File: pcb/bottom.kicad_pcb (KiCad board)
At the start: 2 copper layers, 128.6 x 95.2 mm, 7 parts

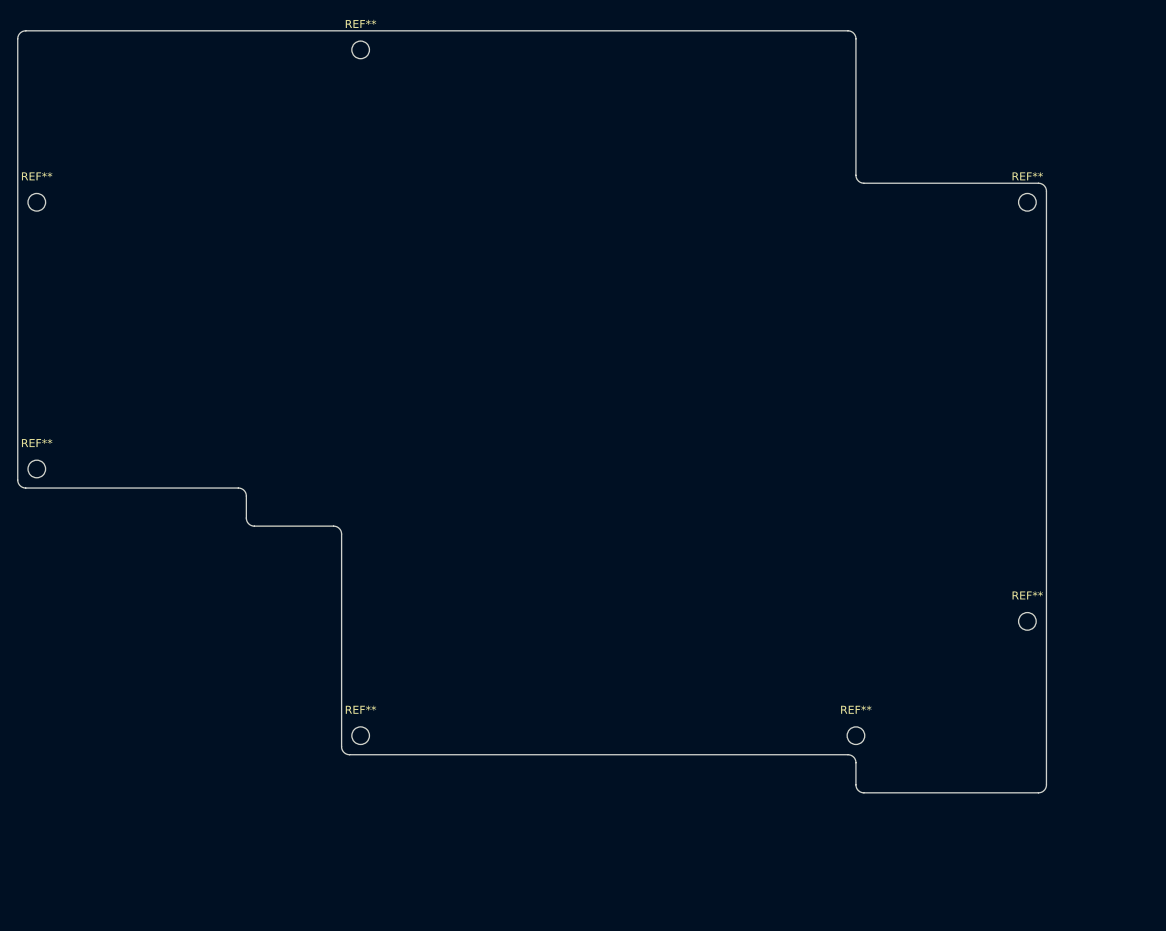
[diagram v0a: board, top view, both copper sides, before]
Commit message: add: pcb and plate garber files
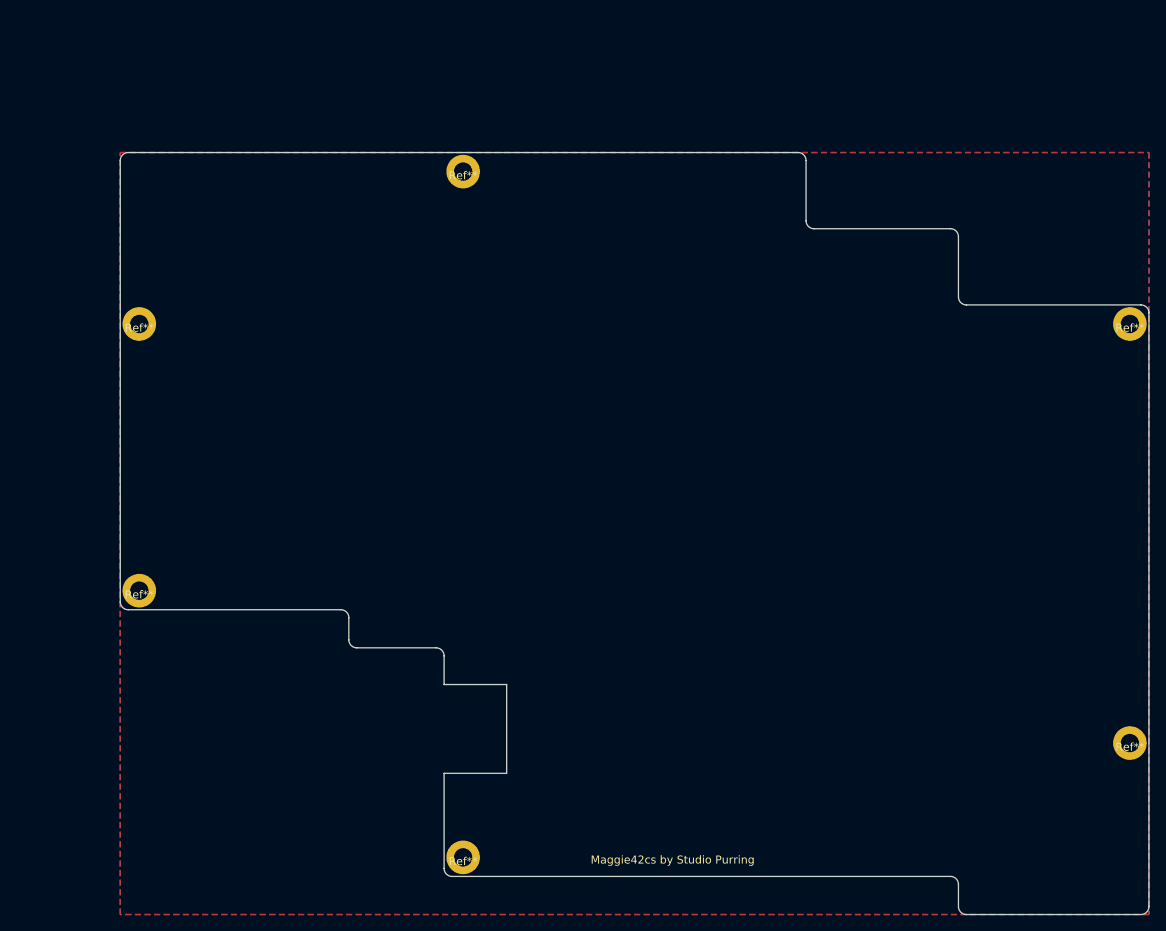
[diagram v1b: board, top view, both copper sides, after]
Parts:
- removed REF** (x7): MountingHole_2.2mm_M2, MountingHole:MountingHole_2.2mm_M2
- added Ref**: Val**, kbd:M2_Hole_TH, F.Cu at (29.5, 50.9)
- added Ref**: Val**, kbd:M2_Hole_TH, F.Cu at (153.3, 50.9)
- added Ref**: Val**, kbd:M2_Hole_TH, F.Cu at (29.5, 84.3)
- added Ref**: Val**, kbd:M2_Hole_TH, F.Cu at (70.0, 117.6)
- added Ref**: Val**, kbd:M2_Hole_TH, F.Cu at (153.3, 103.3)
- added Ref**: Val**, kbd:M2_Hole_TH, F.Cu at (70.0, 31.9)
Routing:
- added copper zone on B.Cu, net GND
- added copper zone on F.Cu, net GND
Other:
- outline, holes or cut-outs redrawn
- board text added: "Maggie42cs by Studio Purring"
